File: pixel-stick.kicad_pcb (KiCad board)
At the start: 2 copper layers, 16.5 x 37.1 mm, 15 parts, among them J2 WS28**, U1 AZ1117-3.3, U2 ESP-01v090, U3 SN74LVC1T45DBV, U4 RT9361A

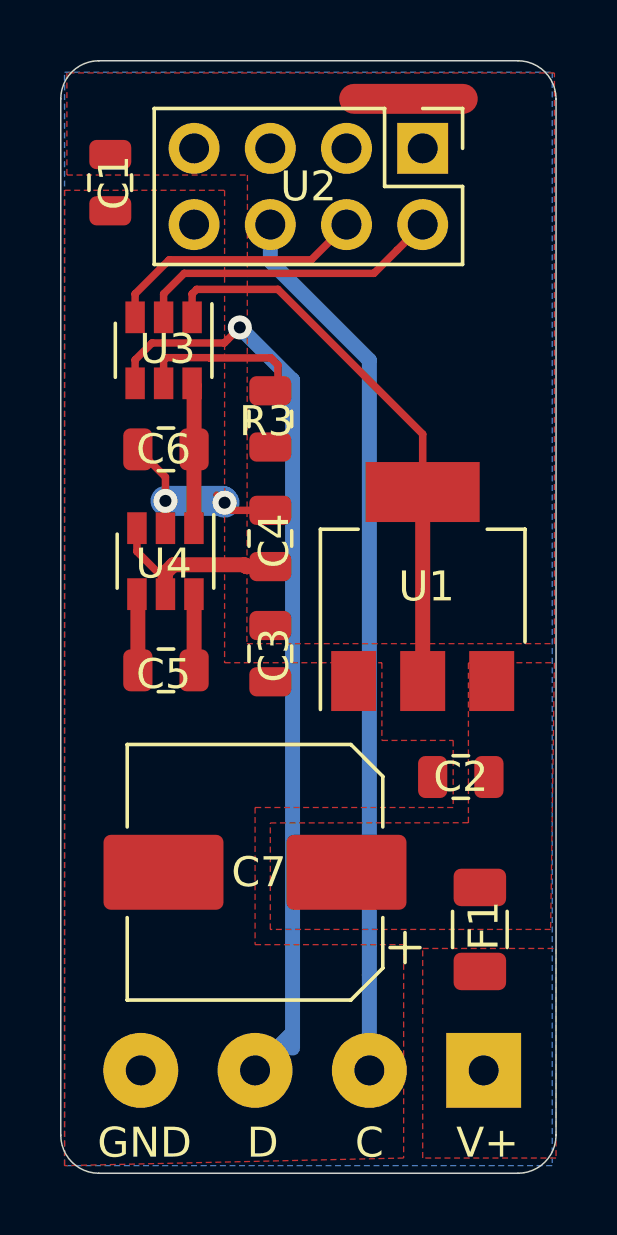
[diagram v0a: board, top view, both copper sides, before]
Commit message: more layer cleanup
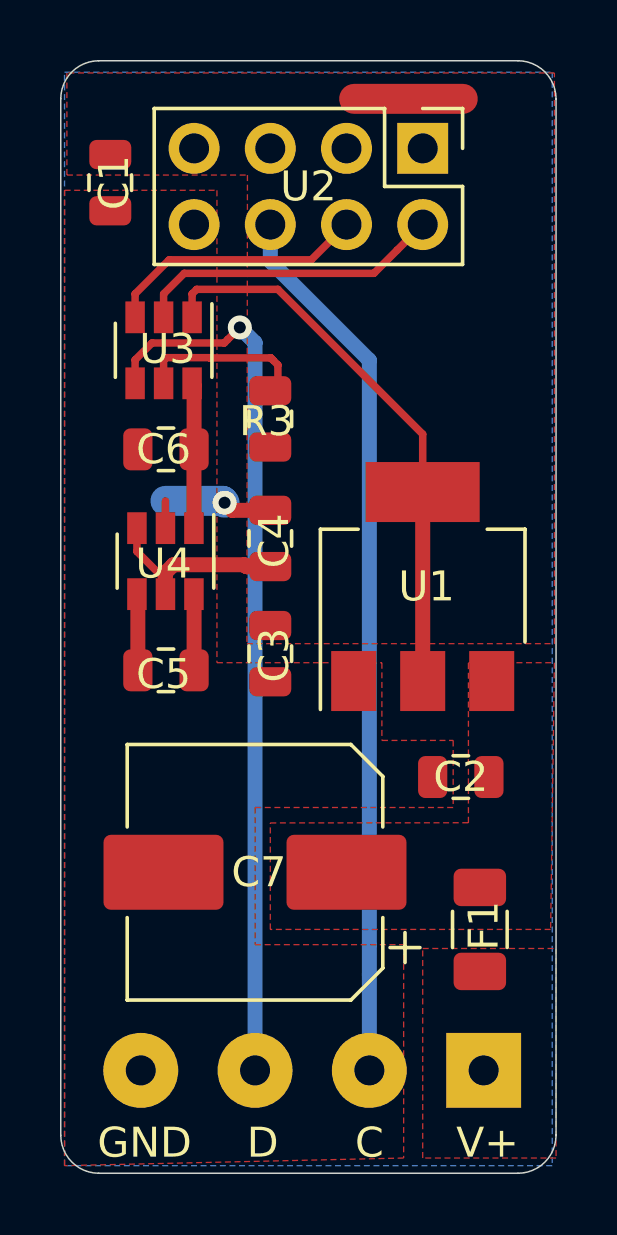
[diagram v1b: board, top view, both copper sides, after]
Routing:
- net GND: track 17.4 -> 14.9 mm, vias 2 -> 1
- net /DATA: track 31.2 -> 29.7 mm
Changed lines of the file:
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@@
     (thickness 1.6)
     (drawings 13)
-    (tracks 66)
+    (tracks 61)
     (zones 0)
     (modules 15)
@@
   )
   (setup
-    (last_trace_width 0.25)
+    (last_trace_width 0.5)
     (user_trace_width 0.5)
     (user_trace_width 1)
@@
   (gr_line (start 43.815 90.678) (end 57.785 90.678) (layer Edge.Cuts) (width 0.05))
   (gr_line (start 42.545 54.864) (end 42.545 89.408) (layer Edge.Cuts) (width 0.05))
-  (segment (start 46.035 67.468) (end 46.035 68.265) (width 0.25) (layer F.Cu) (net 1))
-  (segment (start 45.115 66.548) (end 46.035 67.468) (width 0.25) (layer F.Cu) (net 1))
-  (segment (start 49.53 68.58) (end 48.26 68.58) (width 0.25) (layer F.Cu) (net 1))
-  (segment (start 48.26 68.58) (end 48.006 68.326) (width 0.25) (layer F.Cu) (net 1))
-  (segment (start 48.006 68.326) (end 47.752 68.072) (width 0.25) (layer F.Cu) (net 1))
-  (via (at 48.006 68.326) (size 0.8) (drill 0.4) (layers F.Cu B.Cu) (net 1) (status 1000000))
+  (via (at 48.006 68.326) (size 0.8) (drill 0.4) (layers F.Cu B.Cu) (net 1))
   (segment (start 46.035 68.265) (end 46.035 69.174) (width 0.25) (layer F.Cu) (net 1))
-  (via (at 46.035 68.265) (size 0.8) (drill 0.4) (layers F.Cu B.Cu) (net 1))
   (segment (start 47.945 68.265) (end 48.006 68.326) (width 1) (layer B.Cu) (net 1))
   (segment (start 46.035 68.265) (end 47.945 68.265) (width 1) (layer B.Cu) (net 1))
@@
   (segment (start 52.984989 60.680011) (end 53.760001 59.904999) (width 0.25) (layer F.Cu) (net 1))
   (segment (start 45.974 62.146) (end 45.974 61.366) (width 0.25) (layer F.Cu) (net 1))
+  (segment (start 48.26 68.58) (end 48.006 68.326) (width 0.5) (layer F.Cu) (net 1))
+  (segment (start 49.53 68.58) (end 48.26 68.58) (width 0.5) (layer F.Cu) (net 1))
   (segment (start 45.085 69.954) (end 46.035 70.904) (width 0.25) (layer F.Cu) (net 2))
   (segment (start 46.035 70.904) (end 46.035 71.374) (width 0.25) (layer F.Cu) (net 2))
@@
   (segment (start 52.832 87.249) (end 52.832 84.074) (width 0.5) (layer B.Cu) (net 10))
   (via (at 48.514 62.484) (size 0.8) (drill 0.4) (layers F.Cu B.Cu) (net 11))
-  (segment (start 49.022 87.249) (end 50.271679 85.999321) (width 0.5) (layer B.Cu) (net 11))
   (segment (start 48.114001 62.883999) (end 48.514 62.484) (width 0.25) (layer F.Cu) (net 11))
   (segment (start 47.996999 63.001001) (end 48.114001 62.883999) (width 0.25) (layer F.Cu) (net 11))
@@
   (segment (start 45.024 63.566) (end 45.588999 63.001001) (width 0.25) (layer F.Cu) (net 11))
   (segment (start 45.024 64.346) (end 45.024 63.566) (width 0.25) (layer F.Cu) (net 11))
-  (segment (start 50.271679 64.241679) (end 48.514 62.484) (width 0.5) (layer B.Cu) (net 11))
-  (segment (start 50.271679 86.507321) (end 50.271679 64.241679) (width 0.5) (layer B.Cu) (net 11))
+  (segment (start 49.022 62.992) (end 48.514 62.484) (width 0.5) (layer B.Cu) (net 11))
+  (segment (start 49.022 87.249) (end 49.022 62.992) (width 0.5) (layer B.Cu) (net 11))
   (segment (start 52.832 63.578314) (end 52.832 83.058) (width 0.5) (layer B.Cu) (net 12))
   (segment (start 49.53 60.276314) (end 52.832 63.578314) (width 0.5) (layer B.Cu) (net 12))
@@
     (polygon
       (pts
-        (xy 42.672 57.912) (xy 48.006 57.912) (xy 48.006 73.66) (xy 53.25 73.66) (xy 53.25 76.25)
+        (xy 42.672 57.912) (xy 47.752 57.912) (xy 47.752 73.66) (xy 53.25 73.66) (xy 53.25 76.25)
         (xy 55.626 76.25) (xy 55.626 78.486) (xy 49.022 78.486) (xy 49.022 83.058) (xy 53.975 83.058)
         (xy 53.975 90.17) (xy 42.672 90.424)

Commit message: more power/gnd plane cleanup
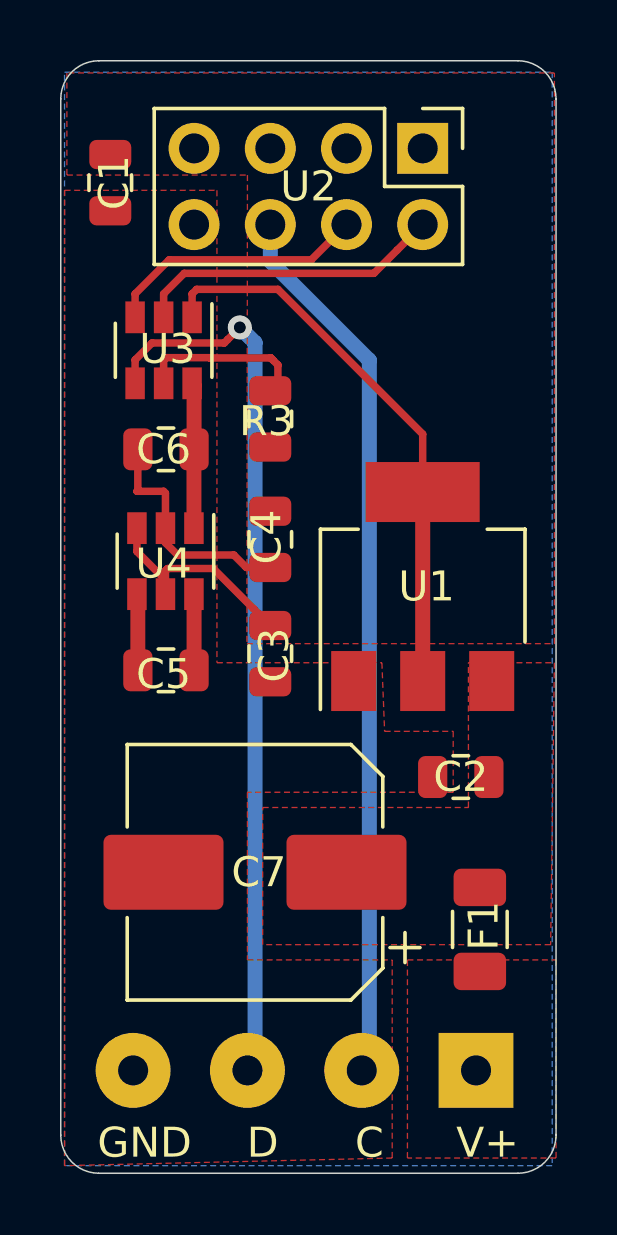
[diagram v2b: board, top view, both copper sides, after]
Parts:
- moved J2 0.25 mm to (56.4, 87.2)
- turned C4 to 270 degrees
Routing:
- net GND: track 14.9 -> 18.3 mm, vias 1 -> 0
- net +3V3: track 29.4 -> 26.5 mm
